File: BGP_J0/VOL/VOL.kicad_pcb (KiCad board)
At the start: 2 copper layers, 25 x 28 mm, 27 parts, among them J1 Conn_01x03_Female, P1 CONN_01X03, P2 CONN_01X02, P3 CONN_01X04, P4 CONN_01X02, Q1 MMBF5457, Q2 MMBF5457

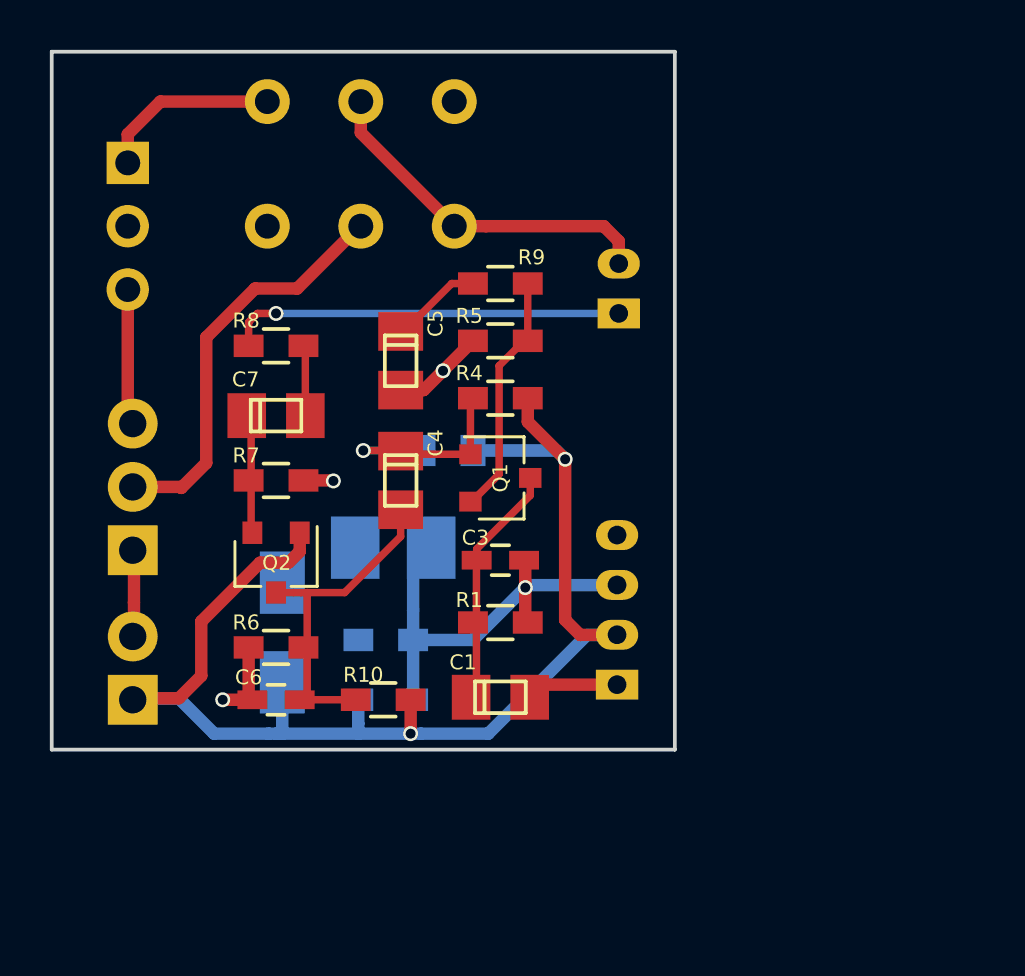
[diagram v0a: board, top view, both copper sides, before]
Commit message: J0 - Panelisation
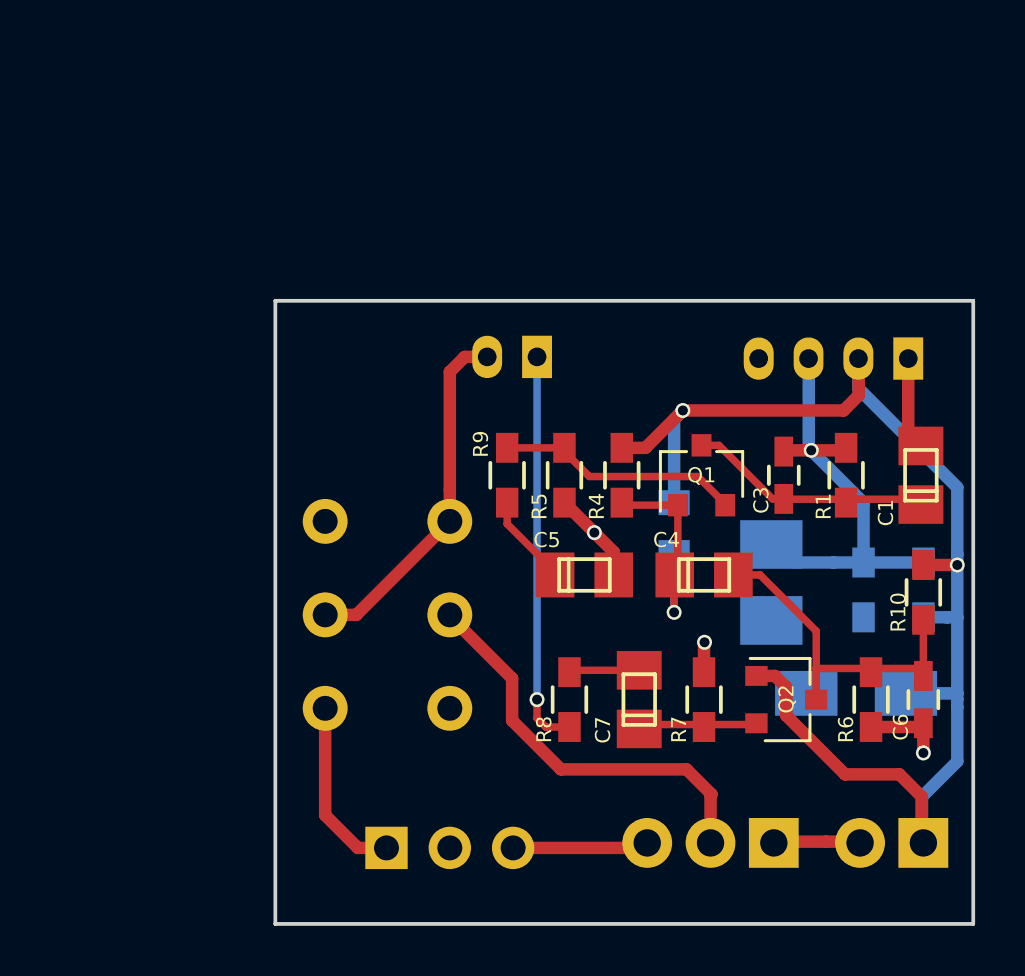
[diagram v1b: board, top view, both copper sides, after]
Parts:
- moved P2 32.2 mm to (172.0, 119.8), turned to 180 degrees
- moved J1 29.4 mm to (150.4, 120.0), turned to 270 degrees
- moved P1 28.3 mm to (166.0, 119.8), turned to 180 degrees
- moved C6 26.0 mm to (172.0, 114.0), turned to 270 degrees
- moved RV2 24.5 mm to (148.0, 114.4), turned to 180 degrees
- moved R6 24.0 mm to (169.9, 114.0), turned to 270 degrees
- moved D1 23.2 mm to (169.3, 113.8), turned to 180 degrees
- moved R10 22.1 mm to (172.0, 109.7), turned to 270 degrees
- moved R2 22.0 mm to (172.0, 109.6), turned to 90 degrees
- moved Q2 21.2 mm to (166.5, 114.0), turned to 0 degrees
- moved R7 19.3 mm to (163.2, 114.0), turned to 90 degrees
- moved R3 19.3 mm to (169.6, 109.6), turned to 270 degrees
- moved C1 19.1 mm to (171.9, 105.0), turned to 270 degrees
- moved C7 18.5 mm to (160.6, 114.0), turned to 270 degrees
- moved R8 18.4 mm to (157.8, 114.0), turned to 90 degrees
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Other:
- board size 25 x 28 mm -> 28 x 25 mm
